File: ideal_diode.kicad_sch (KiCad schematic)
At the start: 5 parts, among them Q11 BSC059N04LS6, U18 LM74700

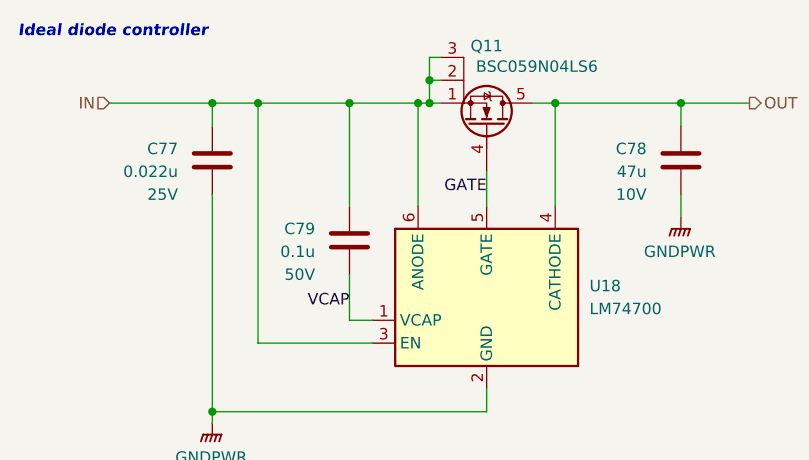
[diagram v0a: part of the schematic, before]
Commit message: Unsure of changes
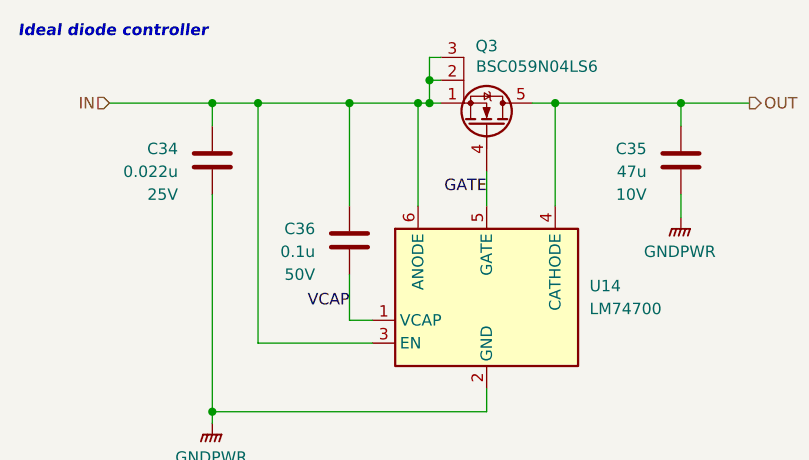
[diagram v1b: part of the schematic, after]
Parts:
- renumbered C77 to C34, C78 to C35, C79 to C36, Q11 to Q3, U18 to U14
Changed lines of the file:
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@@
 		(on_board yes)
 		(dnp no)
-		(property "Reference" "C78"
+		(property "Reference" "C35"
 			(at 121.92 36.8299 0)
 			(effects
@@
 		(on_board yes)
 		(dnp no)
-		(property "Reference" "C77"
+		(property "Reference" "C34"
 			(at 69.85 36.8299 0)
 			(effects
@@
 		(dnp no)
 		(fields_autoplaced yes)
-		(property "Reference" "#PWR0104"
+		(property "Reference" "#PWR095"
 			(at 73.66 72.39 0)
 			(effects
@@
 		(on_board yes)
 		(dnp no)
-		(property "Reference" "C79"
+		(property "Reference" "C36"
 			(at 85.09 45.7199 0)
 			(effects
@@
 		(on_board yes)
 		(dnp no)
-		(property "Reference" "Q11"
+		(property "Reference" "Q3"
 			(at 104.14 25.4 90)
 			(effects
@@
 		(dnp no)
 		(fields_autoplaced yes)
-		(property "Reference" "U18"
+		(property "Reference" "U14"
 			(at 115.57 52.0699 0)
 			(effects
@@
 		(dnp no)
 		(fields_autoplaced yes)
-		(property "Reference" "#PWR0103"
+		(property "Reference" "#PWR094"
 			(at 125.73 49.53 0)
 			(effects
